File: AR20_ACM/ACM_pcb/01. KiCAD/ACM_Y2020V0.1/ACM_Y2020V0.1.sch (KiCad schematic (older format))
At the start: 32 parts, among them J1 TC2030-MCP-NL, P1 Conn_02x15_Odd_Even, Q1 Q_PMOS_DGS, U1 ATmega328PB-AU, U2 MCP25625-x-SS, U3 NCV890430MW50TXG, Y1 16.0Mhz

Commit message: Changelog for 06.10.2019
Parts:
- J1: symbol TC2030-MCP-NL:TC2030-MCP-NL -> ACM_Y2020V0.1-rescue:TC2030-MCP-NL-TC2030-MCP-NL
- LED1: symbol SMLP36RGB2W3R:SMLP36RGB2W3R -> ACM_Y2020V0.1-rescue:SMLP36RGB2W3R-SMLP36RGB2W3R
- U3: symbol NCV890430MW50TXG:NCV890430MW50TXG -> ACM_Y2020V0.1-rescue:NCV890430MW50TXG-NCV890430MW50TXG
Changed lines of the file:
@@
 $EndDescr
 $Comp
-L TC2030-MCP-NL:TC2030-MCP-NL J1
+L ACM_Y2020V0.1-rescue:TC2030-MCP-NL-TC2030-MCP-NL J1
 U 1 1 5D389624
 P 1075 1400
@@
 $EndComp
 $Comp
-L SMLP36RGB2W3R:SMLP36RGB2W3R LED1
+L ACM_Y2020V0.1-rescue:SMLP36RGB2W3R-SMLP36RGB2W3R LED1
 U 1 1 5D41B8EC
 P 8575 1450
@@
 	1750 2525 575  2525
 $Comp
-L NCV890430MW50TXG:NCV890430MW50TXG U3
+L ACM_Y2020V0.1-rescue:NCV890430MW50TXG-NCV890430MW50TXG U3
 U 1 1 5D46D022
 P 5525 5800

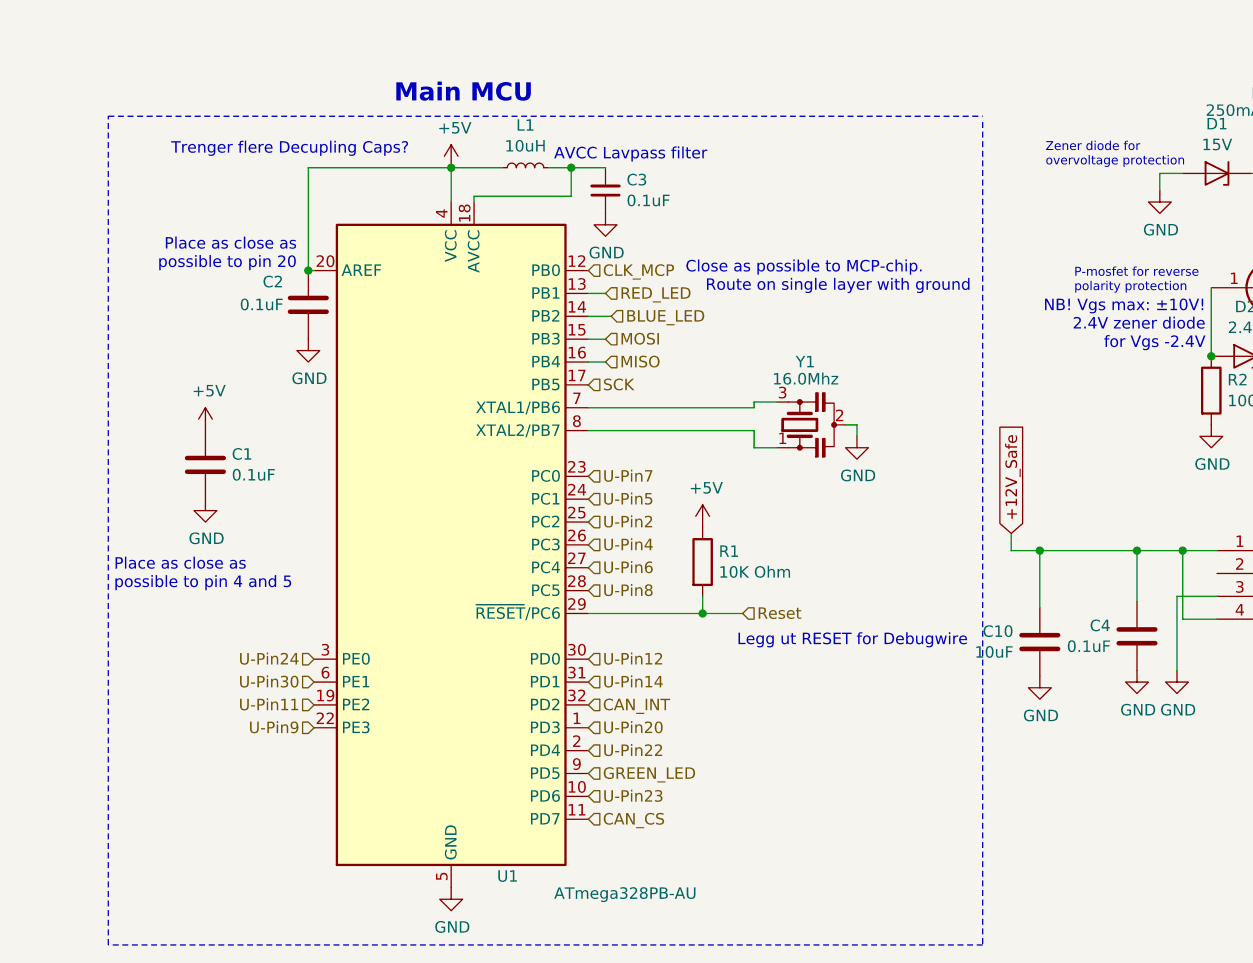
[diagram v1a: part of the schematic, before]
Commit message: Changelog for 06.10.2019
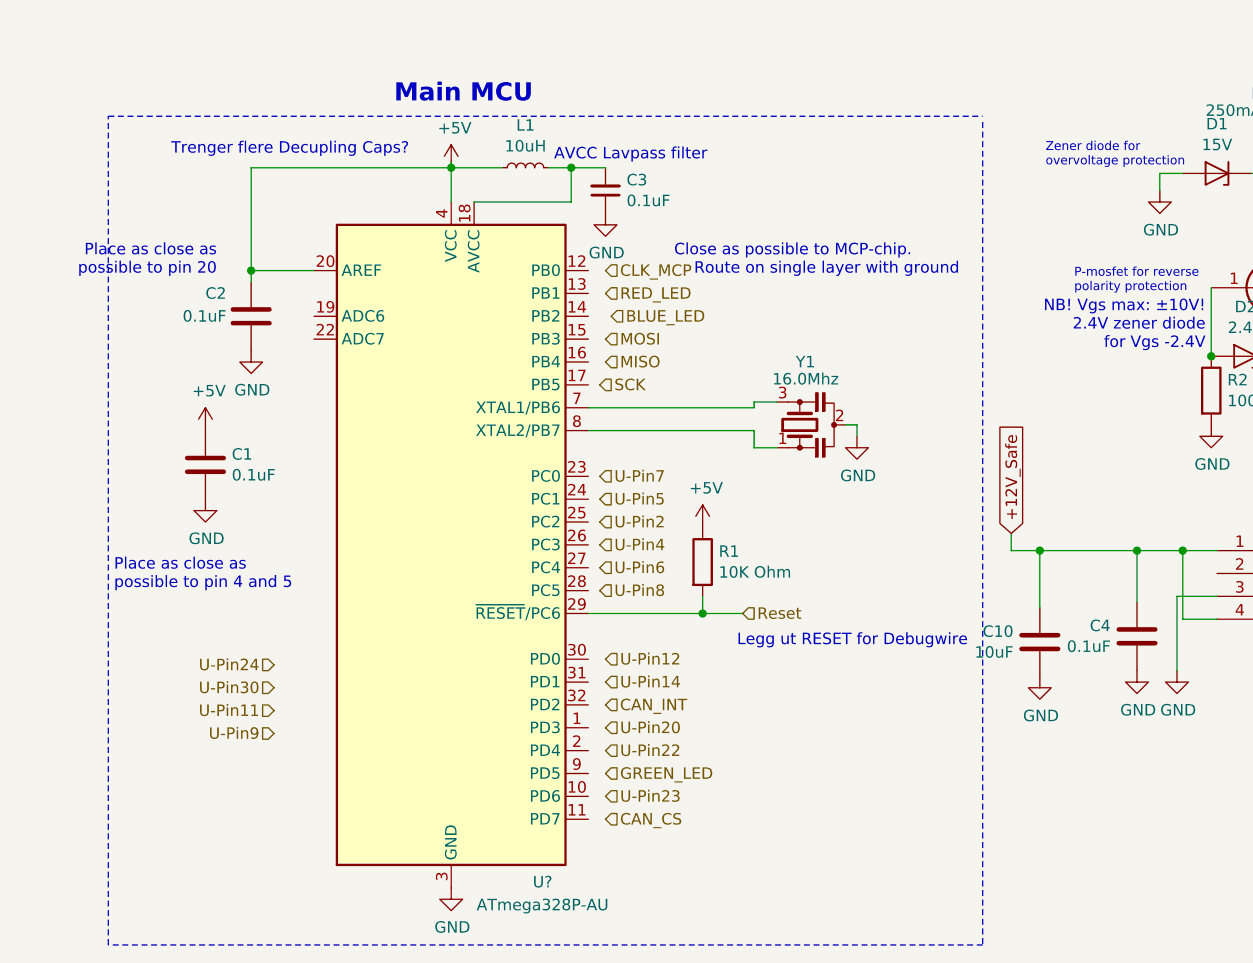
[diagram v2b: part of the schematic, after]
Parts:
- removed U1: ATmega328PB-AU, Package_QFP:TQFP-32_7x7mm_P0.8mm, symbol MCU_Microchip_ATmega:ATmega328PB-AU
- added U?: ATmega328P-AU, Package_QFP:TQFP-32_7x7mm_P0.8mm, symbol MCU_Microchip_ATmega:ATmega328P-AU
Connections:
- net +5V: now also U?.20 (AREF), U?.4 (VCC), U?.6 (VCC)
- net GND: now also U?.21 (GND), U?.3 (GND), U?.5 (GND)
- net Reset: now also U?.29 (~RESET~/PC6)
- net at C3.2, L1.2: now also U?.18 (AVCC)
- net at Y1.3: now also U?.7 (XTAL1/PB6)
- net at Y1.1: now also U?.8 (XTAL2/PB7)
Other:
- moved on the sheet: C2
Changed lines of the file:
@@
 	1    0    0    -1
 $EndComp
-Wire Wire Line
-	2175 4125 2175 4275
 $Comp
 L Device:C C1
@@
 	1    0    0    -1
 $EndComp
-Wire Wire Line
-	2775 6075 3275 6075
 $Comp
 L power:+5V #PWR09
@@
 	1    0    0    -1
 $EndComp
-Text HLabel 2775 6975 2    50   Input ~ 0
+Text HLabel 2850 6975 2    50   Input ~ 0
 CAN_CS
 Text HLabel 8875 4500 0    50   Input ~ 0
@@
 	1    0    0    -1
 $EndComp
-Text HLabel 2775 6475 2    50   Input ~ 0
+Text HLabel 2850 6475 2    50   Input ~ 0
 CAN_INT
 Text HLabel 8875 5600 0    50   Input ~ 0
@@
 Wire Wire Line
 	10175 1450 10175 1375
-Text HLabel 2775 6775 2    50   Input ~ 0
+Text HLabel 2850 6775 2    50   Input ~ 0
 GREEN_LED
 $Comp
@@
 Wire Wire Line
 	6025 1875 6425 1875
-Text HLabel 1575 6275 0    50   Input ~ 0
+Text HLabel 1400 6300 0    50   Input ~ 0
 U-Pin24
-Text HLabel 1575 6375 0    50   Input ~ 0
+Text HLabel 1400 6400 0    50   Input ~ 0
 U-Pin30
-Text HLabel 1575 6475 0    50   Input ~ 0
+Text HLabel 1400 6500 0    50   Input ~ 0
 U-Pin11
-Text HLabel 1575 6575 0    50   Input ~ 0
+Text HLabel 1400 6600 0    50   Input ~ 0
 U-Pin9
-Text HLabel 2775 6675 2    50   Input ~ 0
+Text HLabel 2850 6675 2    50   Input ~ 0
 U-Pin22
-Text HLabel 2775 6575 2    50   Input ~ 0
+Text HLabel 2850 6575 2    50   Input ~ 0
 U-Pin20
-Text HLabel 2775 6375 2    50   Input ~ 0
+Text HLabel 2850 6375 2    50   Input ~ 0
 U-Pin14
-Text HLabel 2775 6275 2    50   Input ~ 0
+Text HLabel 2850 6275 2    50   Input ~ 0
 U-Pin12
-Connection ~ 3275 6075
 Wire Wire Line
 	3275 6075 3275 6000
-Text HLabel 2775 5975 2    50   Input ~ 0
+Text HLabel 2825 5975 2    50   Input ~ 0
 U-Pin8
-Text HLabel 2775 5875 2    50   Input ~ 0
+Text HLabel 2825 5875 2    50   Input ~ 0
 U-Pin6
-Text HLabel 2775 5775 2    50   Input ~ 0
+Text HLabel 2825 5775 2    50   Input ~ 0
 U-Pin4
-Text HLabel 2775 5675 2    50   Input ~ 0
+Text HLabel 2825 5675 2    50   Input ~ 0
 U-Pin2
-Text HLabel 2775 5575 2    50   Input ~ 0
-U-Pin5
-Text HLabel 2775 5475 2    50   Input ~ 0
+Text HLabel 2825 5475 2    50   Input ~ 0
 U-Pin7
 Text HLabel 10775 3900 2    50   Input ~ 0
@@
 Wire Wire Line
 	3500 5275 2775 5275
-Text HLabel 2775 6875 2    50   Input ~ 0
+Text HLabel 2850 6875 2    50   Input ~ 0
 U-Pin23
 Text HLabel 5900 1575 2    50   Input ~ 0
@@
 AVCC Lavpass filter
 Wire Wire Line
-	2275 4275 2275 4250
-Wire Wire Line
-	2275 4250 2700 4250
-Wire Wire Line
-	2700 4250 2700 4125
-Wire Wire Line
 	2850 4125 2700 4125
 Connection ~ 2700 4125
@@
 	2400 4125 2175 4125
 Connection ~ 2175 4125
-Wire Wire Line
-	1550 4125 2175 4125
-Text Notes 1500 4575 2    50   ~ 0
+Text Notes 1150 4600 2    50   ~ 0
 Place as close as \npossible to pin 20
-Connection ~ 1550 4575
 $Comp
 L power:GND #PWR03
 U 1 1 5D434DF4
-P 1550 4875
-F 0 "#PWR03" H 1550 4625 50  0001 C CNN
-F 1 "GND" H 1555 4702 50  0000 C CNN
-F 2 "" H 1550 4875 50  0001 C CNN
-F 3 "" H 1550 4875 50  0001 C CNN
-	1    1550 4875
+P 1300 4925
+F 0 "#PWR03" H 1300 4675 50  0001 C CNN
+F 1 "GND" H 1305 4752 50  0000 C CNN
+F 2 "" H 1300 4925 50  0001 C CNN
+F 3 "" H 1300 4925 50  0001 C CNN
+	1    1300 4925
 	1    0    0    -1
 $EndComp
@@
 L Device:C C2
 U 1 1 5D434DE8
-P 1550 4725
-F 0 "C2" H 1350 4825 50  0000 L CNN
-F 1 "0.1uF" H 1250 4725 50  0000 L CNN
-F 2 "Capacitor_SMD:C_0402_1005Metric" H 1588 4575 50  0001 C CNN
-F 3 "~" H 1550 4725 50  0001 C CNN
-	1    1550 4725
-	1    0    0    -1
-$EndComp
-Wire Wire Line
-	1550 4575 1550 4125
-Wire Wire Line
-	1575 4575 1550 4575
-Wire Wire Line
-	2775 4975 2850 4975
-Wire Wire Line
-	2775 4875 2850 4875
-Wire Wire Line
-	2775 4775 2875 4775
-Wire Wire Line
-	2775 4675 2850 4675
+P 1300 4775
+F 0 "C2" H 1100 4875 50  0000 L CNN
+F 1 "0.1uF" H 1000 4775 50  0000 L CNN
+F 2 "Capacitor_SMD:C_0402_1005Metric" H 1338 4625 50  0001 C CNN
+F 3 "~" H 1300 4775 50  0001 C CNN
+	1    1300 4775
+	1    0    0    -1
+$EndComp
 Wire Wire Line
 	3500 5175 3500 5150
@@
 Wire Wire Line
 	3500 5150 3600 5150
-Text Notes 3200 4675 0    50   ~ 0
+Text Notes 3150 4600 0    50   ~ 0
 Close as possible to MCP-chip.\n    Route on single layer with ground
-Text HLabel 2775 4575 2    50   Input ~ 0
+Text HLabel 2850 4575 2    50   Input ~ 0
 CLK_MCP
-$Comp
-L MCU_Microchip_ATmega:ATmega328PB-AU U1
-U 1 1 5D38D7A6
-P 2175 5775
-F 0 "U1" H 2375 4325 50  0000 L CNN
-F 1 "ATmega328PB-AU" H 2625 4250 50  0000 L CNN
-F 2 "Package_QFP:TQFP-32_7x7mm_P0.8mm" H 2175 5775 50  0001 C CIN
-F 3 "http://ww1.microchip.com/downloads/en/DeviceDoc/40001906C.pdf" H 2175 5775 50  0001 C CNN
-F 4 "https://no.farnell.com/microchip/atmega328pb-au/mcu-8bit-atmega-20mhz-tqfp-32/dp/2523203?st=ATMEGA328p" H 2175 5775 50  0001 C CNN "Farnell"
-	1    2175 5775
-	1    0    0    -1
-$EndComp
 $Comp
 L Device:Resonator_Small Y1
@@
 Text HLabel 2850 4975 2    50   Input ~ 0
 MISO
-Text HLabel 2775 5075 2    50   Input ~ 0
+Text HLabel 2825 5075 2    50   Input ~ 0
 SCK
 $Comp
@@
 Wire Wire Line
 	6825 6075 7600 6075
+$Comp
+L MCU_Microchip_ATmega:ATmega328P-AU U?
+U 1 1 5D9A1492
+P 2175 5775
+F 0 "U?" H 2575 4300 50  0000 C CNN
+F 1 "ATmega328P-AU" H 2575 4200 50  0000 C CNN
+F 2 "Package_QFP:TQFP-32_7x7mm_P0.8mm" H 2175 5775 50  0001 C CIN
+F 3 "http://ww1.microchip.com/downloads/en/DeviceDoc/ATmega328_P%20AVR%20MCU%20with%20picoPower%20Technology%20Data%20Sheet%2040001984A.pdf" H 2175 5775 50  0001 C CNN
+	1    2175 5775
+	1    0    0    -1
+$EndComp
+Text HLabel 2825 5575 2    50   Input ~ 0
+U-Pin5
+Wire Wire Line
+	2175 4100 2175 4125
+Wire Wire Line
+	2175 4125 2175 4275
+Wire Wire Line
+	2275 4275 2700 4275
+Wire Wire Line
+	2700 4125 2700 4275
+Wire Wire Line
+	2775 6075 3275 6075
+Connection ~ 3275 6075
+Wire Wire Line
+	1575 4575 1300 4575
+Wire Wire Line
+	1300 4575 1300 4625
+Wire Wire Line
+	1300 4575 1300 4125
+Wire Wire Line
+	1300 4125 2175 4125
+Connection ~ 1300 4575
 $EndSCHEMATC
